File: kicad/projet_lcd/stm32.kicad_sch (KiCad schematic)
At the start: 24 parts, among them Y2 NI, Y3 32.768KHz

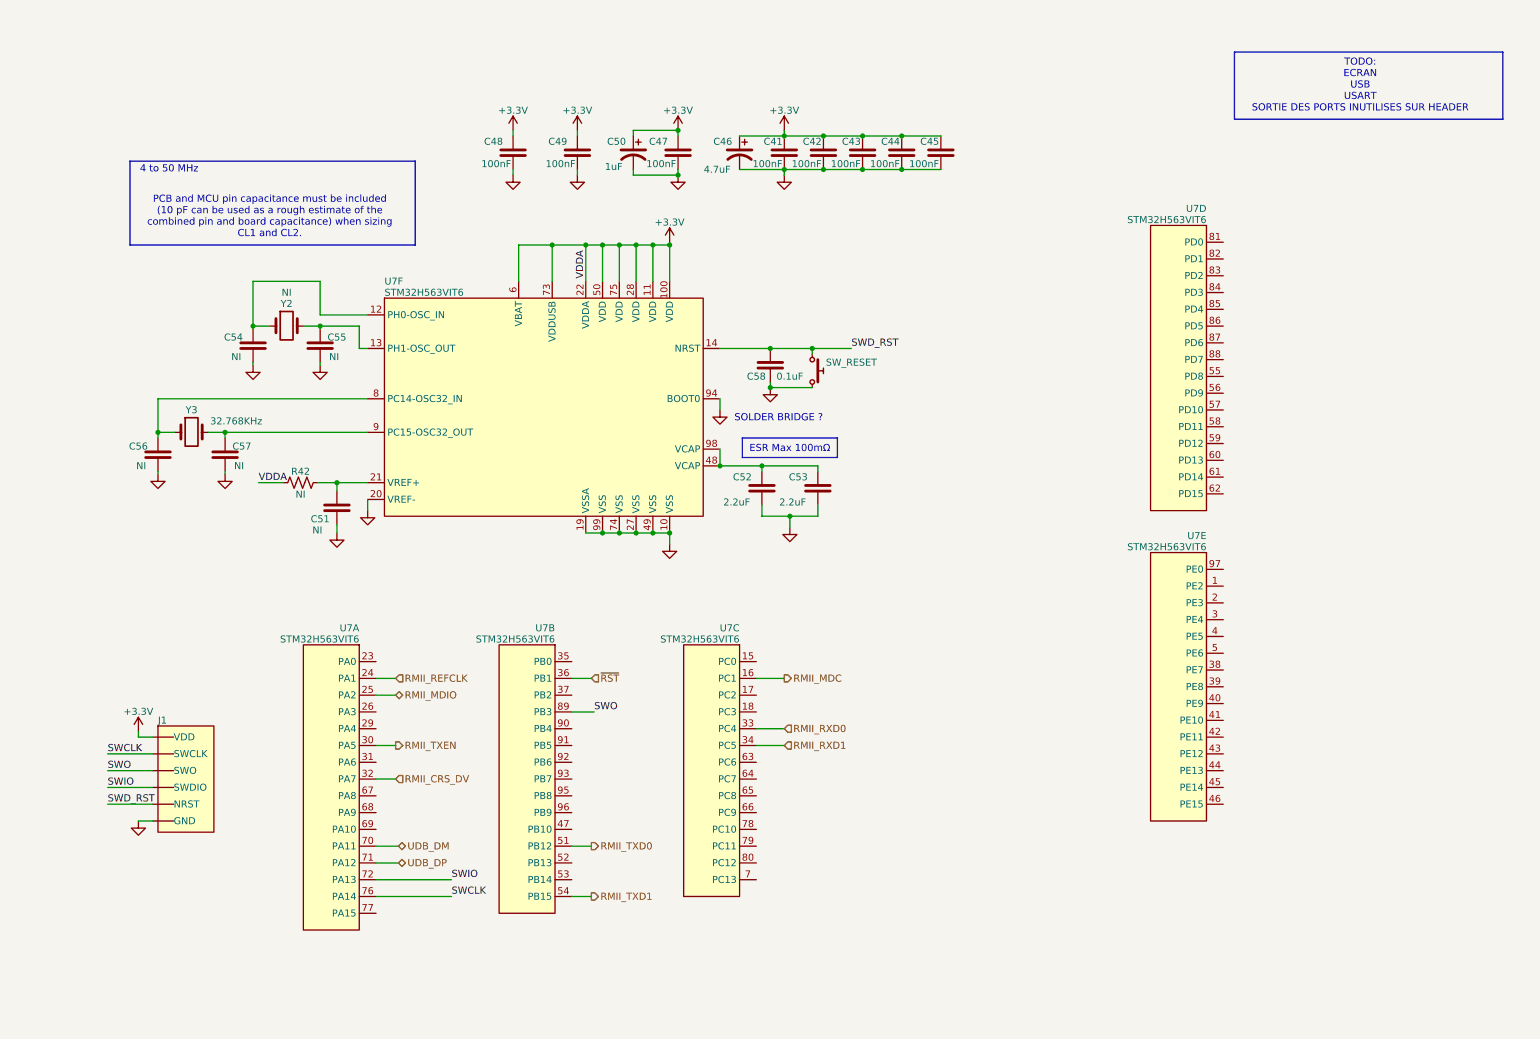
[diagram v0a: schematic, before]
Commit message: EOD
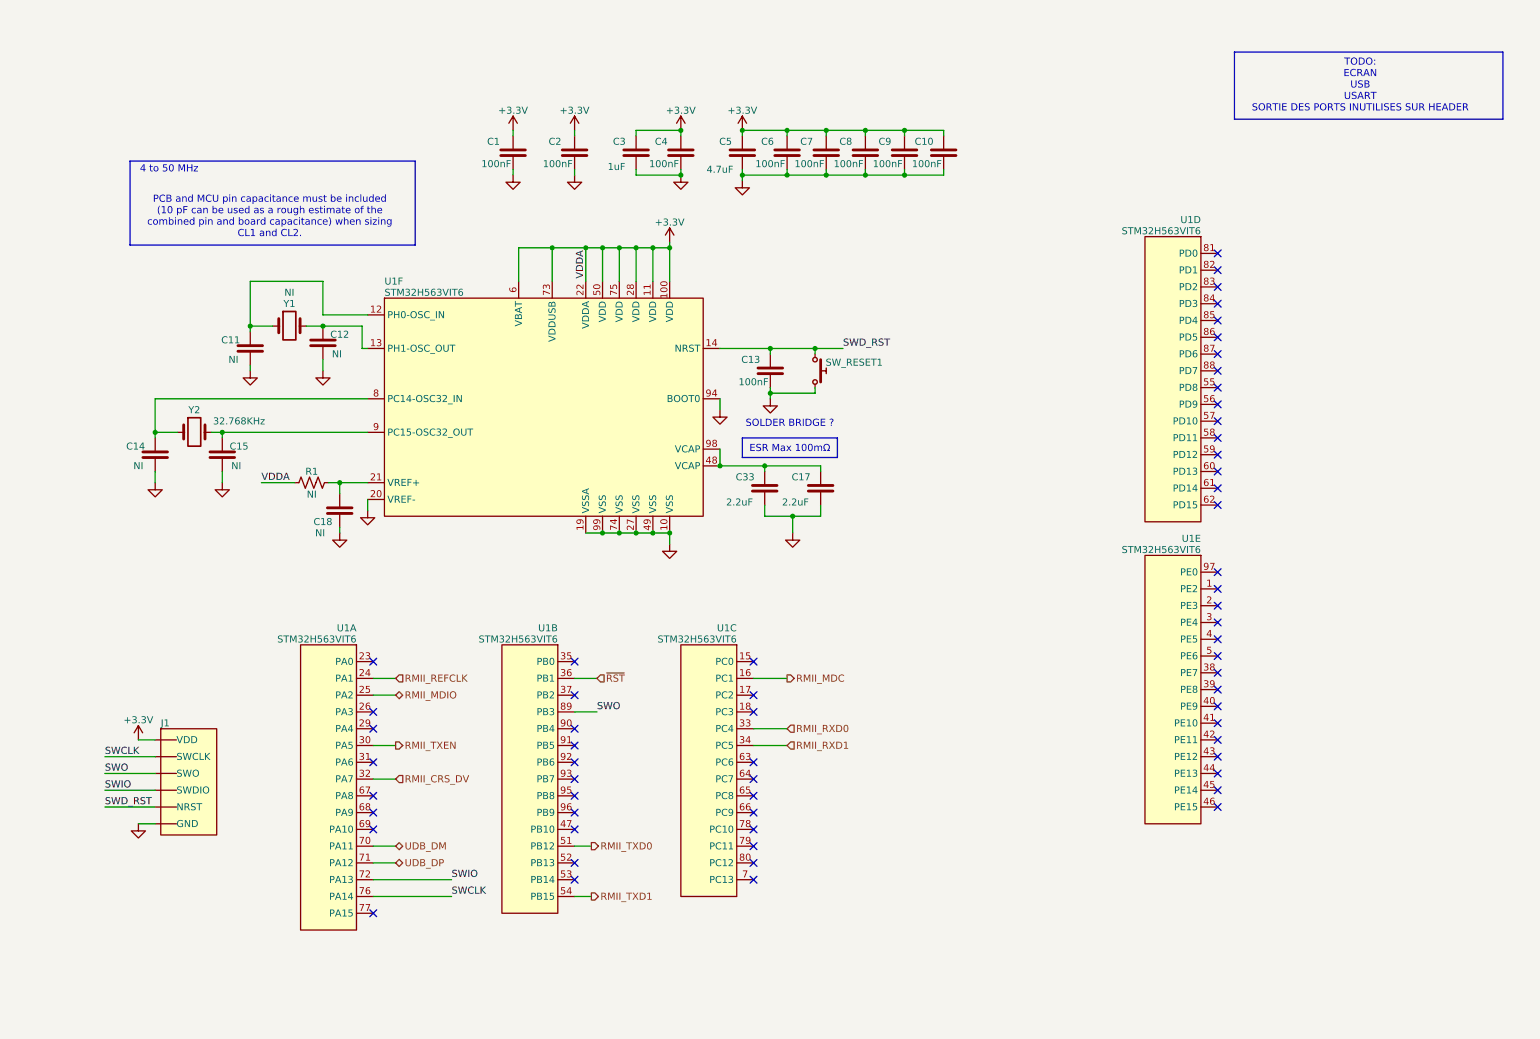
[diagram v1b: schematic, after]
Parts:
- removed C41, C42, C43, C44, C45, C47, C49: 100nF, symbol Generics:C
- removed C52: 2.2uF, symbol Generics:C
- removed C58: 0.1uF, symbol Generics:C
- added C10, C13, C2, C4, C6, C7, C8, C9: 100nF, Generics:C_0603, symbol Generics:C
- added C33: 2.2uF, Generics:C_0402, symbol Generics:C
- C1: renamed from C48; footprint (none) -> Generics:C_0603; LCSC Part # (none) -> C14663
- C17: renamed from C53; footprint (none) -> Generics:C_0402; LCSC Part # (none) -> C12530
- C3: renamed from C50; footprint (none) -> Generics:C_0603; symbol Generics:C_Polarized -> Generics:C; LCSC Part # (none) -> C15849
- C5: renamed from C46; footprint (none) -> Generics:C_0603; symbol Generics:C_Polarized -> Generics:C; LCSC Part # (none) -> C19666
- renumbered C54 to C11, C55 to C12, C56 to C14, C57 to C15, C51 to C18, R42 to R1, SW_RESET to SW_RESET1, U7 to U1, Y2 to Y1, Y3 to Y2
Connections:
- net +3.3V: now also C3.2, C5.2, C10.2, C2.2, C4.2, C6.2, C7.2, C8.2, C9.2; no longer C3.P, C5.P
- net GND: now also C3.1, C5.1, C10.1, C13.1, C2.1, C33.1, C4.1, C6.1, C7.1, C8.1, C9.1; no longer C3.N, C5.N
- net SWD_RST: now also C13.2
- net at C17.2, U1.48 (VCAP), U1.98 (VCAP): now also C33.2
- no-connect marks 0 -> 61
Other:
- moved on the sheet: C11, C12, C18, J1, R1, U1D, U1E

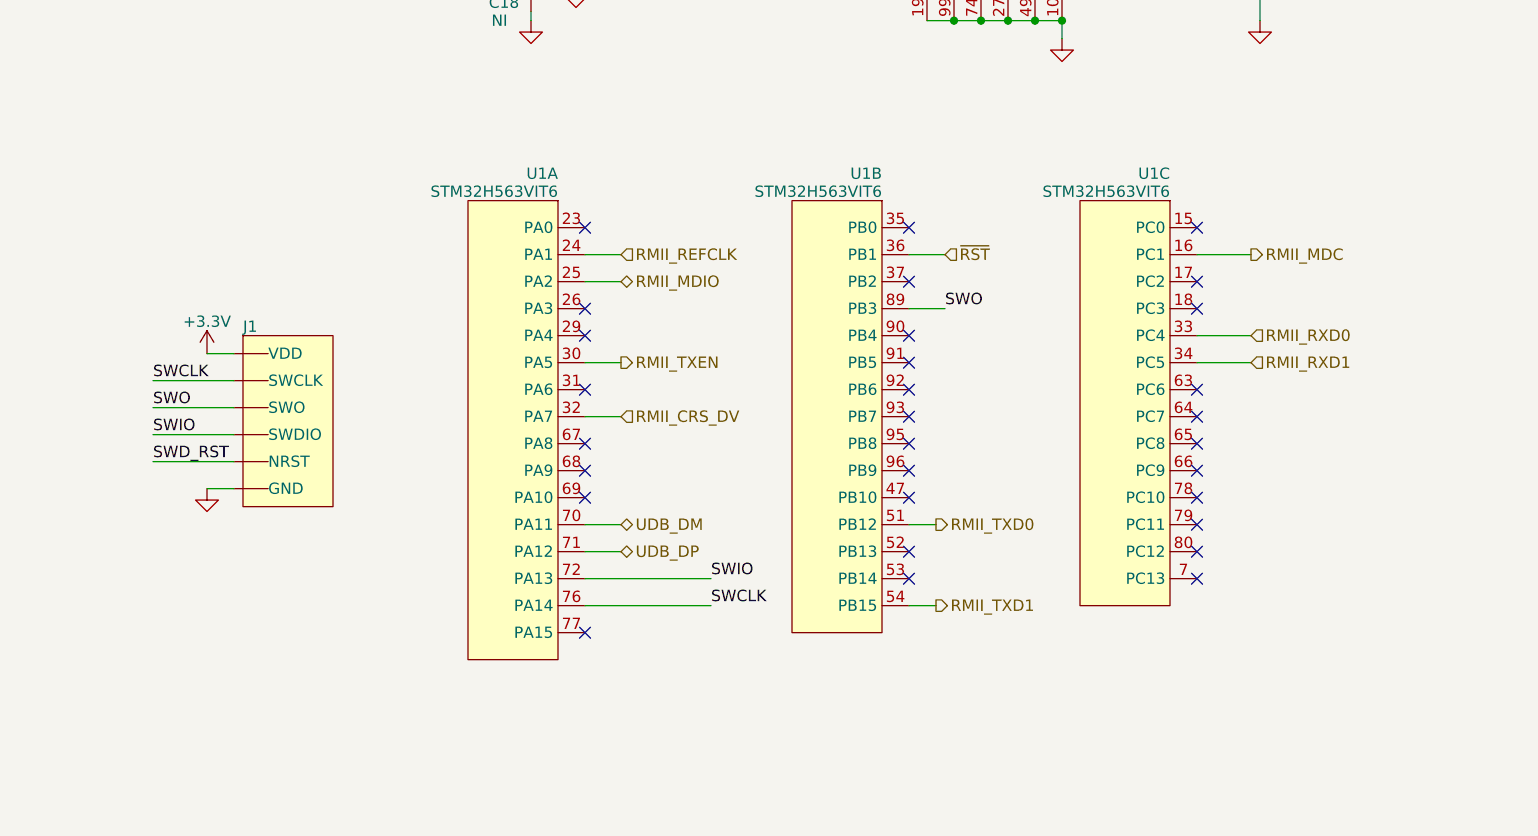
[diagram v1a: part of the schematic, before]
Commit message: EOD
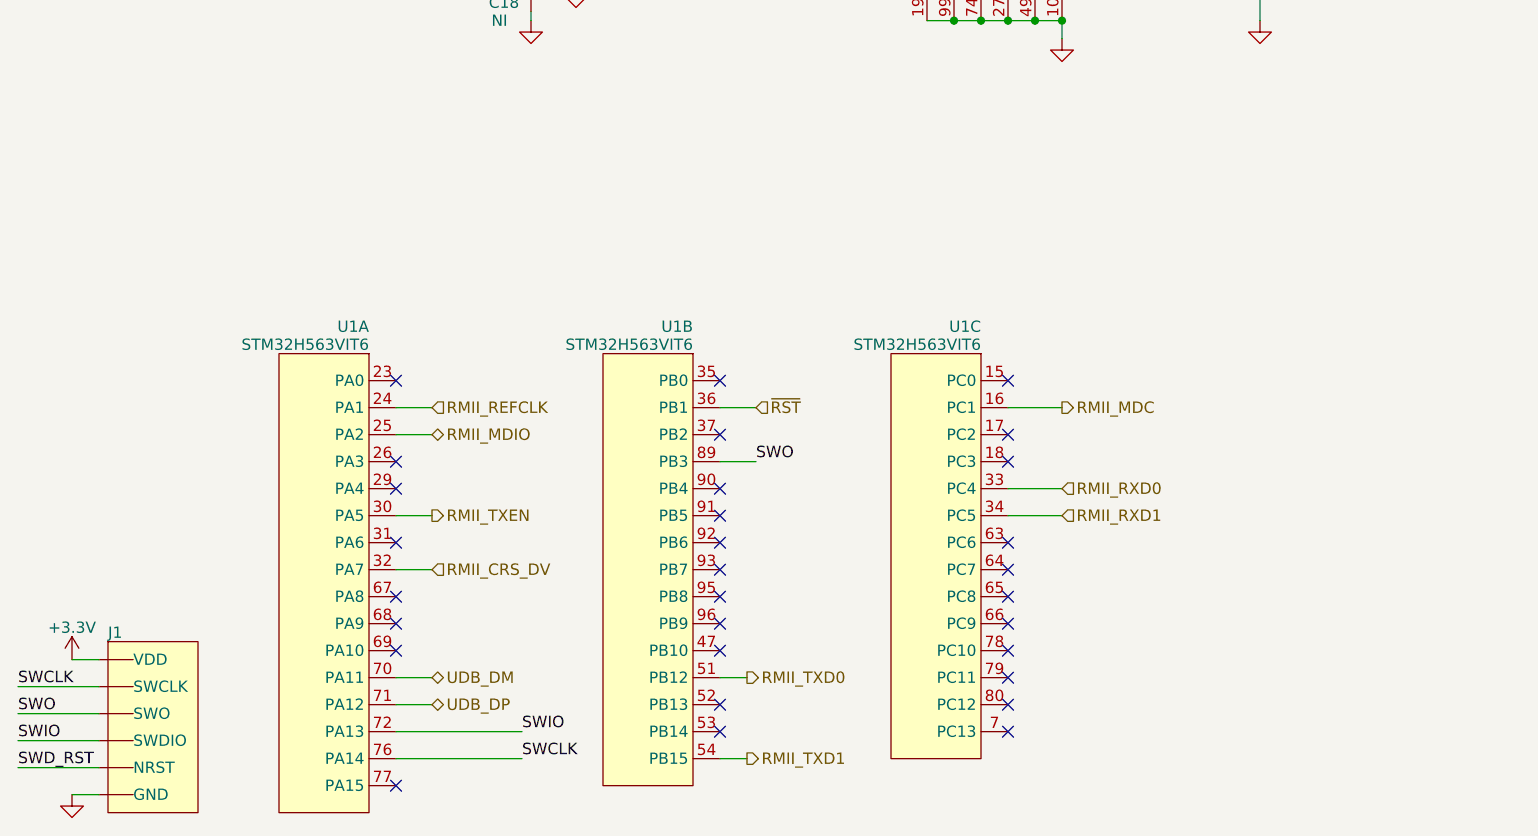
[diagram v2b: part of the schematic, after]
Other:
- moved on the sheet: J1, U1A, U1B, U1C
